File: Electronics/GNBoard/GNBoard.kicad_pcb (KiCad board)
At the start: 2 copper layers, 78.1 x 54.6 mm, 47 parts, among them K1 IR1, K10 IR4, K11 CNY_1, K12 CNY_2, K13 CNY_3, K14 CNY_4, K15 CNY_5, K16 CNY_6, K2 IR2, K3 SERVO_1, K4 SERVO_2, K5 SERVO_3, K6 SERVO_4, K7 SERVO_5, K8 SERVO_6, K9 IR3, P1 Battery, P2 CONN_5, P3 Spk, P4 I2C_1, P5 I2C_2, P6 DHT_Conn, SW1 PowerSwitch, SW2 SW_PUSH, SW3 SW_PUSH, U1 LM2576

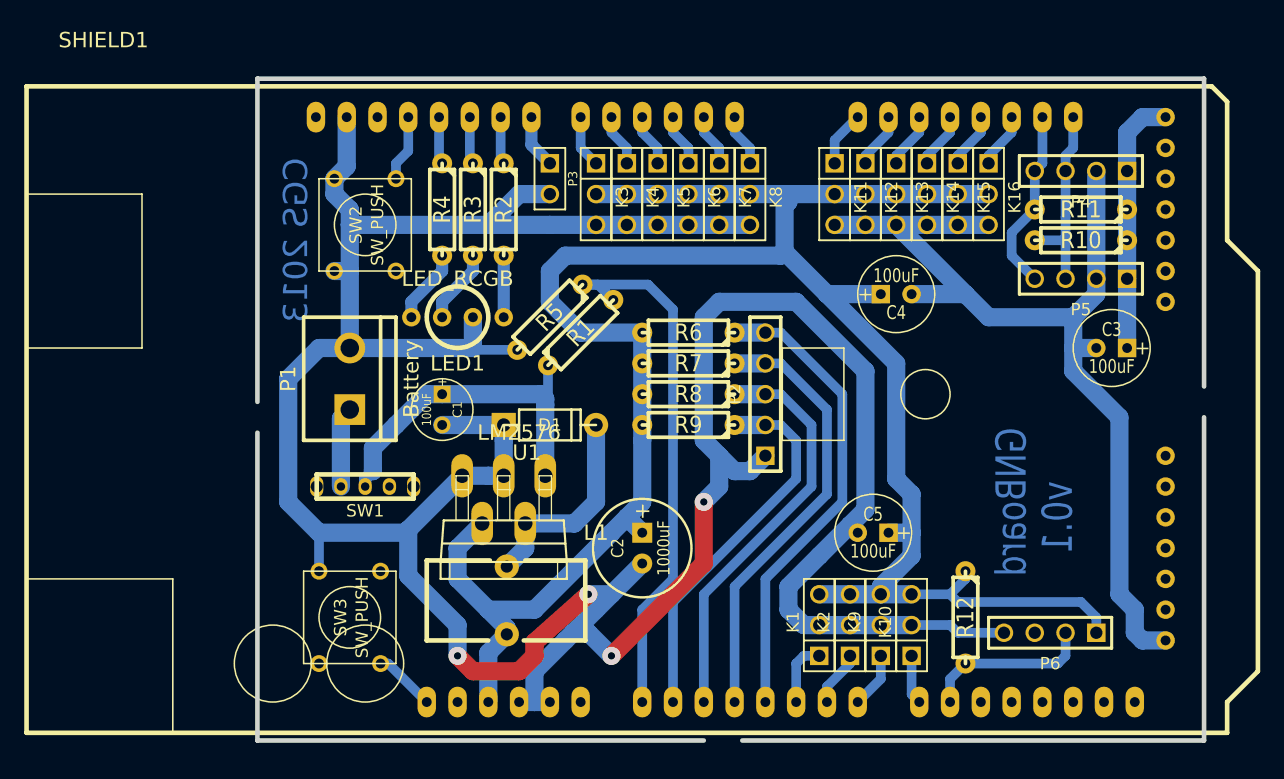
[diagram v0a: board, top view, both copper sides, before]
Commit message: Improvements for the GNBoard
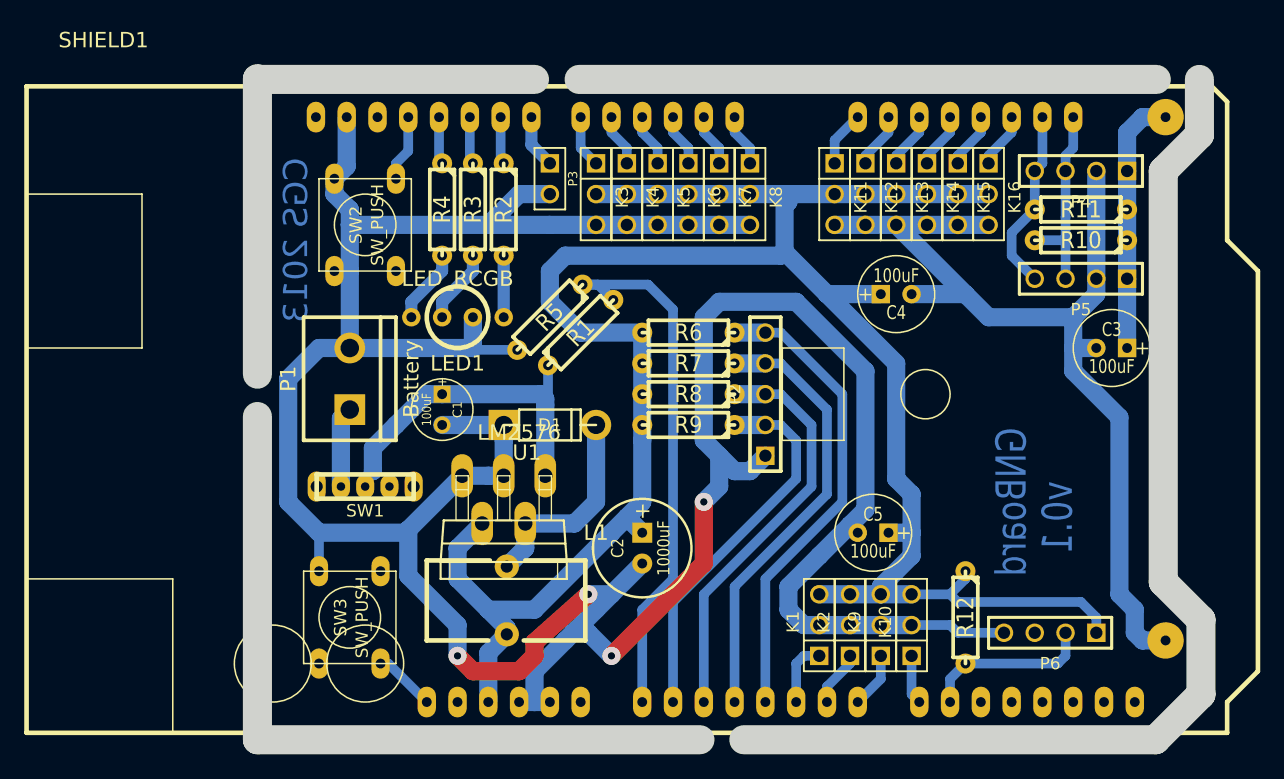
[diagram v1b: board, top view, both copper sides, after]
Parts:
- SW1: footprint MICROSWITCH_SPST -> SWITCH_3Pin
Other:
- board size 78.1 x 54.6 mm -> 77.9 x 54.5 mm
